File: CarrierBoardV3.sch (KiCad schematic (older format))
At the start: 95 parts, among them J1 USB_B_Micro, J10 Conn_02x26_Odd_Even, J11 SW1-12V_SHUNT, J12 SW9-3V3_SHUNT, J13 SW5-5V_SHUNT, J2 Conn_02x09_Odd_Even, J3 Barrel_Jack, J4 TX2iConnctor, J5 Conn_01x03_Male, J6 Conn_02x04_Odd_Even, J7 Conn_02x03_Odd_Even, J8 Conn_02x26_Odd_Even, J9 Conn_01x03_Male, U1 MAX3221, U2 FT232RQ, U3 MSATA-Socket, U4 TXB0104PW, U5 TXB0104PW, U6 MPM3620, U7 LP38851LINREG, U8 MPM3620

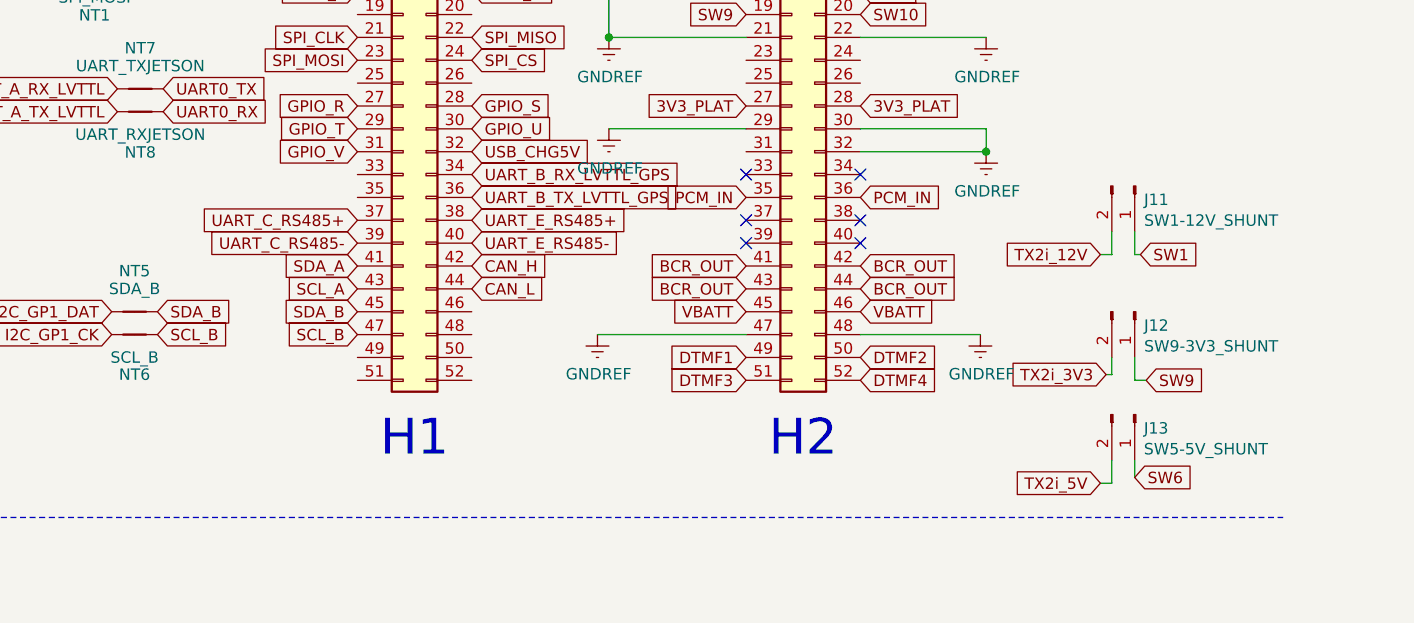
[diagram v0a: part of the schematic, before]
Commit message: Finished Ready for FAB
S/N:0C137_V3_SP19
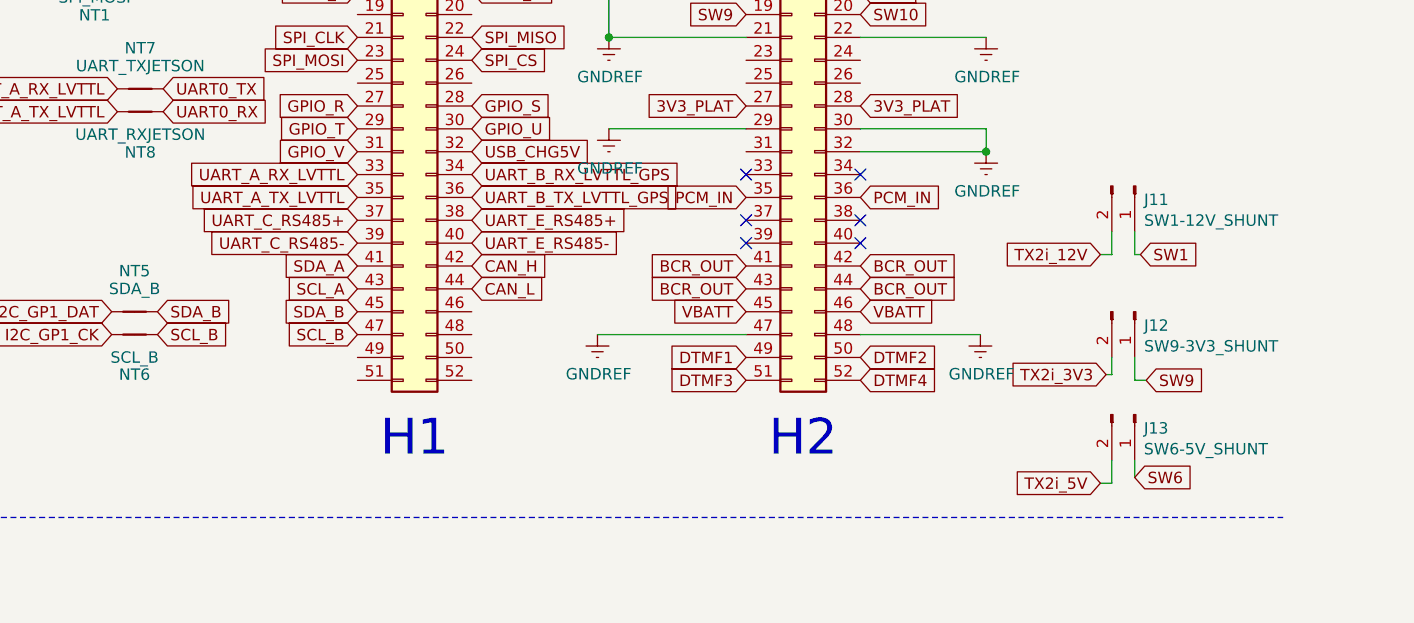
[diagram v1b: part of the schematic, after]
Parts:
- J13: value SW5-5V_SHUNT -> SW6-5V_SHUNT
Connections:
- net UART_A_RX_LVTTL: now also J8.33 (Pin_33)
- net UART_A_TX_LVTTL: now also J8.35 (Pin_35)
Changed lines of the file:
@@
 P 22250 7800
 F 0 "J13" V 22310 7840 50  0000 L CNN
-F 1 "SW5-5V_SHUNT" V 22401 7840 50  0000 L CNN
+F 1 "SW6-5V_SHUNT" V 22401 7840 50  0000 L CNN
 F 2 "Jumper:SolderJumper-2_P1.3mm_Open_Pad1.0x1.5mm" H 22250 7800 50  0001 C CNN
 F 3 "~" H 22250 7800 50  0001 C CNN
@@
 	1    0    0    1
 $EndComp
+Text GLabel 18850 6750 0    50   Input ~ 0
+UART_A_RX_LVTTL
+Text GLabel 18850 6850 0    50   Input ~ 0
+UART_A_TX_LVTTL
 $EndSCHEMATC
